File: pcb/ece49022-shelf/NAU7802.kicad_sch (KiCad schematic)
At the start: 12 parts, among them IC1 NAU7802

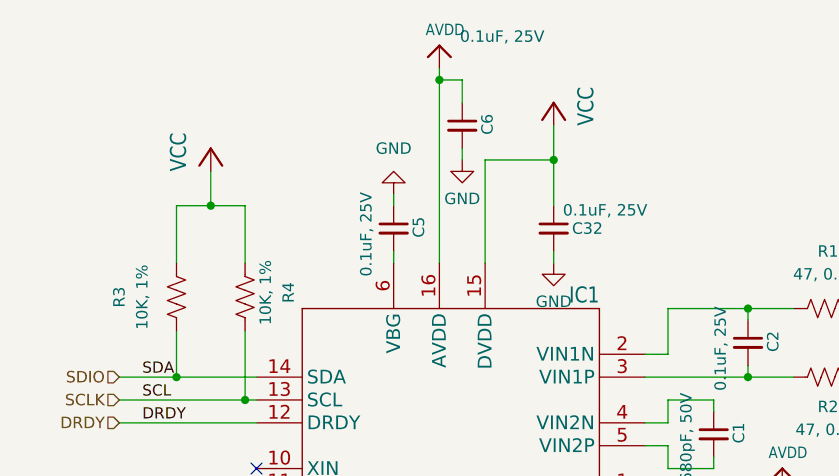
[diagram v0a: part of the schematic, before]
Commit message: working n board
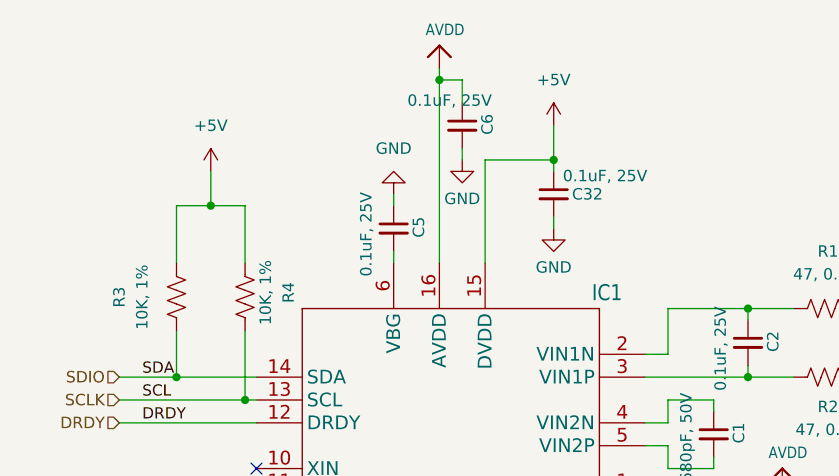
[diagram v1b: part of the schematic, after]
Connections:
- net VCC is gone; now on net +5V: C32.1, IC1.15 (DVDD), R3.2, R4.2
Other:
- moved on the sheet: C32
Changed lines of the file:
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@@
 	(wire
 		(pts
-			(xy 147.32 82.55) (xy 147.32 87.63)
+			(xy 147.32 82.55) (xy 147.32 83.82)
 		)
 		(stroke
@@
 	(wire
 		(pts
-			(xy 147.32 92.71) (xy 147.32 93.98)
+			(xy 147.32 88.9) (xy 147.32 90.17)
 		)
 		(stroke
@@
 	(symbol
 		(lib_id "power:GND")
-		(at 147.32 93.98 0)
+		(at 147.32 90.17 0)
 		(unit 1)
 		(exclude_from_sim no)
@@
 		(dnp no)
 		(property "Reference" "#PWR056"
-			(at 147.32 100.33 0)
+			(at 147.32 96.52 0)
 			(effects
 				(font
@@
 		)
 		(property "Value" "GND"
-			(at 147.32 98.298 0)
+			(at 147.32 94.488 0)
 			(effects
 				(font
@@
 		)
 		(property "Footprint" ""
-			(at 147.32 93.98 0)
+			(at 147.32 90.17 0)
 			(effects
 				(font
@@
 		)
 		(property "Datasheet" ""
-			(at 147.32 93.98 0)
+			(at 147.32 90.17 0)
 			(effects
 				(font
@@
 		)
 		(property "Description" "Power symbol creates a global label with name \"GND\" , ground"
-			(at 147.32 93.98 0)
+			(at 147.32 90.17 0)
 			(effects
 				(font
@@
 				(path "/cb6cb1b4-c151-4aa2-8cd7-5430288cfa02/fb213d7f-28bb-4d6d-ba03-4017b4d07db5"
 					(reference "#PWR056")
-					(unit 1)
-				)
-			)
-		)
-	)
-	(symbol
-		(lib_id "NAU7802-eagle-import:VCC")
-		(at 109.22 81.28 0)
-		(unit 1)
-		(exclude_from_sim no)
-		(in_bom yes)
-		(on_board yes)
-		(dnp no)
-		(property "Reference" "#P+2"
-			(at 109.22 81.28 0)
-			(effects
-				(font
-					(size 1.27 1.27)
-				)
-				(hide yes)
-			)
-		)
-		(property "Value" "VCC"
-			(at 106.68 83.82 90)
-			(effects
-				(font
-					(size 1.778 1.5113)
-				)
-				(justify left bottom)
-			)
-		)
-		(property "Footprint" ""
-			(at 109.22 81.28 0)
-			(effects
-				(font
-					(size 1.27 1.27)
-				)
-				(hide yes)
-			)
-		)
-		(property "Datasheet" ""
-			(at 109.22 81.28 0)
-			(effects
-				(font
-					(size 1.27 1.27)
-				)
-				(hide yes)
-			)
-		)
-		(property "Description" ""
-			(at 109.22 81.28 0)
-			(effects
-				(font
-					(size 1.27 1.27)
-				)
-				(hide yes)
-			)
-		)
-		(pin "1"
-		)
-		(instances
-			(project ""
-				(path "/cb6cb1b4-c151-4aa2-8cd7-5430288cfa02/fb213d7f-28bb-4d6d-ba03-4017b4d07db5"
-					(reference "#P+2")
-					(unit 1)
-				)
-			)
-			(project ""
-				(path "/f46caa08-94e3-4c42-8462-81738f26da11"
-					(reference "#P+2")
 					(unit 1)
 				)
@@
 				(path "/cb6cb1b4-c151-4aa2-8cd7-5430288cfa02/fb213d7f-28bb-4d6d-ba03-4017b4d07db5"
 					(reference "#U$01")
+					(unit 1)
+				)
+			)
+		)
+	)
+	(symbol
+		(lib_id "power:+5V")
+		(at 109.22 83.82 0)
+		(unit 1)
+		(exclude_from_sim no)
+		(in_bom yes)
+		(on_board yes)
+		(dnp no)
+		(fields_autoplaced yes)
+		(property "Reference" "#PWR057"
+			(at 109.22 87.63 0)
+			(effects
+				(font
+					(size 1.27 1.27)
+				)
+				(hide yes)
+			)
+		)
+		(property "Value" "+5V"
+			(at 109.22 78.74 0)
+			(effects
+				(font
+					(size 1.27 1.27)
+				)
+			)
+		)
+		(property "Footprint" ""
+			(at 109.22 83.82 0)
+			(effects
+				(font
+					(size 1.27 1.27)
+				)
+				(hide yes)
+			)
+		)
+		(property "Datasheet" ""
+			(at 109.22 83.82 0)
+			(effects
+				(font
+					(size 1.27 1.27)
+				)
+				(hide yes)
+			)
+		)
+		(property "Description" "Power symbol creates a global label with name \"+5V\""
+			(at 109.22 83.82 0)
+			(effects
+				(font
+					(size 1.27 1.27)
+				)
+				(hide yes)
+			)
+		)
+		(pin "1"
+		)
+		(instances
+			(project "ece49022-shelf"
+				(path "/cb6cb1b4-c151-4aa2-8cd7-5430288cfa02/fb213d7f-28bb-4d6d-ba03-4017b4d07db5"
+					(reference "#PWR057")
 					(unit 1)
 				)
@@
 		)
 		(property "Value" "0.1uF, 25V"
-			(at 136.906 68.834 0)
+			(at 131.064 75.946 0)
 			(effects
 				(font
@@
 	)
 	(symbol
-		(lib_id "NAU7802-eagle-import:VCC")
-		(at 147.32 76.2 0)
-		(mirror y)
-		(unit 1)
-		(exclude_from_sim no)
-		(in_bom yes)
-		(on_board yes)
-		(dnp no)
-		(property "Reference" "#P+7"
-			(at 147.32 76.2 0)
-			(effects
-				(font
-					(size 1.27 1.27)
-				)
-				(hide yes)
-			)
-		)
-		(property "Value" "VCC"
-			(at 149.86 78.74 90)
-			(effects
-				(font
-					(size 1.778 1.5113)
-				)
-				(justify left bottom)
-			)
-		)
-		(property "Footprint" ""
-			(at 147.32 76.2 0)
-			(effects
-				(font
-					(size 1.27 1.27)
-				)
-				(hide yes)
-			)
-		)
-		(property "Datasheet" ""
-			(at 147.32 76.2 0)
-			(effects
-				(font
-					(size 1.27 1.27)
-				)
-				(hide yes)
-			)
-		)
-		(property "Description" ""
-			(at 147.32 76.2 0)
-			(effects
-				(font
-					(size 1.27 1.27)
-				)
-				(hide yes)
-			)
-		)
-		(pin "1"
-		)
-		(instances
-			(project ""
-				(path "/cb6cb1b4-c151-4aa2-8cd7-5430288cfa02/fb213d7f-28bb-4d6d-ba03-4017b4d07db5"
-					(reference "#P+7")
-					(unit 1)
-				)
-			)
-			(project ""
-				(path "/f46caa08-94e3-4c42-8462-81738f26da11"
-					(reference "#P+7")
-					(unit 1)
-				)
-			)
-		)
-	)
-	(symbol
 		(lib_id "Device:C_Small")
 		(at 168.91 102.87 0)
@@
 		(dnp no)
 		(property "Reference" "IC1"
-			(at 152.4 96.52 0)
+			(at 154.94 96.266 0)
 			(effects
 				(font
@@
 	(symbol
 		(lib_id "Device:C_Small")
-		(at 147.32 90.17 0)
+		(at 147.32 86.36 0)
 		(unit 1)
 		(exclude_from_sim no)
@@
 		(dnp no)
 		(property "Reference" "C32"
-			(at 149.352 90.17 0)
+			(at 149.352 86.36 0)
 			(effects
 				(font
@@
 		)
 		(property "Value" "0.1uF, 25V"
-			(at 148.336 88.138 0)
+			(at 148.336 84.328 0)
 			(effects
 				(font
@@
 		)
 		(property "Footprint" "Capacitor_SMD:C_0402_1005Metric"
-			(at 147.32 90.17 0)
+			(at 147.32 86.36 0)
 			(effects
 				(font
@@
 		)
 		(property "Datasheet" "~"
-			(at 147.32 90.17 0)
+			(at 147.32 86.36 0)
 			(effects
 				(font
@@
 		)
 		(property "Description" "0402B104K250HI"
-			(at 147.32 90.17 0)
+			(at 147.32 86.36 0)
 			(effects
 				(font
@@
 					(unit 1)
 				)
+			)
+		)
+	)
+	(symbol
+		(lib_id "power:+5V")
+		(at 147.32 78.74 0)
+		(unit 1)
+		(exclude_from_sim no)
+		(in_bom yes)
+		(on_board yes)
+		(dnp no)
+		(fields_autoplaced yes)
+		(property "Reference" "#PWR058"
+			(at 147.32 82.55 0)
+			(effects
+				(font
+					(size 1.27 1.27)
+				)
+				(hide yes)
+			)
+		)
+		(property "Value" "+5V"
+			(at 147.32 73.66 0)
+			(effects
+				(font
+					(size 1.27 1.27)
+				)
+			)
+		)
+		(property "Footprint" ""
+			(at 147.32 78.74 0)
+			(effects
+				(font
+					(size 1.27 1.27)
+				)
+				(hide yes)
+			)
+		)
+		(property "Datasheet" ""
+			(at 147.32 78.74 0)
+			(effects
+				(font
+					(size 1.27 1.27)
+				)
+				(hide yes)
+			)
+		)
+		(property "Description" "Power symbol creates a global label with name \"+5V\""
+			(at 147.32 78.74 0)
+			(effects
+				(font
+					(size 1.27 1.27)
+				)
+				(hide yes)
+			)
+		)
+		(pin "1"
+		)
+		(instances
+			(project "ece49022-shelf"
+				(path "/cb6cb1b4-c151-4aa2-8cd7-5430288cfa02/fb213d7f-28bb-4d6d-ba03-4017b4d07db5"
+					(reference "#PWR058")
+					(unit 1)
+				)
